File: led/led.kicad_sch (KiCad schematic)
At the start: 0 parts

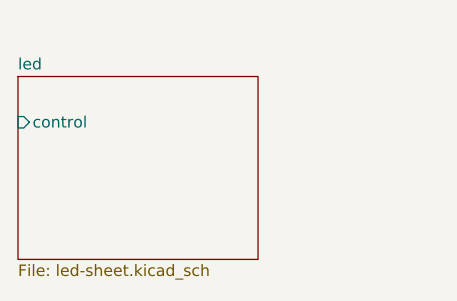
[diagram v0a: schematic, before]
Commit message: baseline
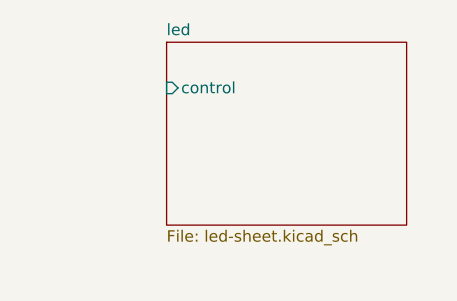
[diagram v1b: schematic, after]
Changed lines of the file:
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@@
 (kicad_sch (version 20201015) (generator eeschema)
   (paper "A4")
-  (sheet (at 135.255 81.915) (size 26.67 20.32)
+  (sheet (at 151.765 78.105) (size 26.67 20.32)
     (stroke (width 0.001) (type solid) (color 132 0 132 1))
     (fill (color 255 255 255 0.0000))
-    (property "Sheet name" "led" (id 0) (at 135.255 81.2791 0)
+    (property "Sheet name" "led" (id 0) (at 151.765 77.4691 0)
       (effects (font (size 1.27 1.27)) (justify left bottom))
     )
-    (property "Sheet file" "led-sheet.kicad_sch" (id 1) (at 135.255 102.7439 0)
+    (property "Sheet file" "led-sheet.kicad_sch" (id 1) (at 151.765 98.9339 0)
       (effects (font (size 1.27 1.27)) (justify left top))
     )
-    (pin "control" input (at 135.255 86.995 180)
+    (pin "control" input (at 151.765 83.185 180)
       (effects (font (size 1.27 1.27)) (justify left))
     )
@@
   )
   (symbol_instances
+    (path "/f6f98991-c174-4124-bca3-675ab210d740/7c882403-2416-47bd-8142-e59dd72b85d2"
+      (reference "#FLG?") (unit 1) (value "PWR_FLAG") (footprint "")
+    )
+    (path "/f6f98991-c174-4124-bca3-675ab210d740/c3651b6a-2384-4d61-a9c6-16a6611a5d34"
+      (reference "#FLG?") (unit 1) (value "PWR_FLAG") (footprint "")
+    )
     (path "/f6f98991-c174-4124-bca3-675ab210d740/301a2811-f3c7-43e4-b172-f5cfe8cfc596"
       (reference "#PWR05") (unit 1) (value "+3V3") (footprint "")
